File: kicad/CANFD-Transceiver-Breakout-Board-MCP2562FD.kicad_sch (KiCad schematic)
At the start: 15 parts, among them IC1 MCP2562FD-E_SN, K1 HEADER_MALE_6X1, K2 HEADER_MALE_6X1, K3 TERMINAL_KF235-5.0-2P, U3 ATA6561-GAQW-N

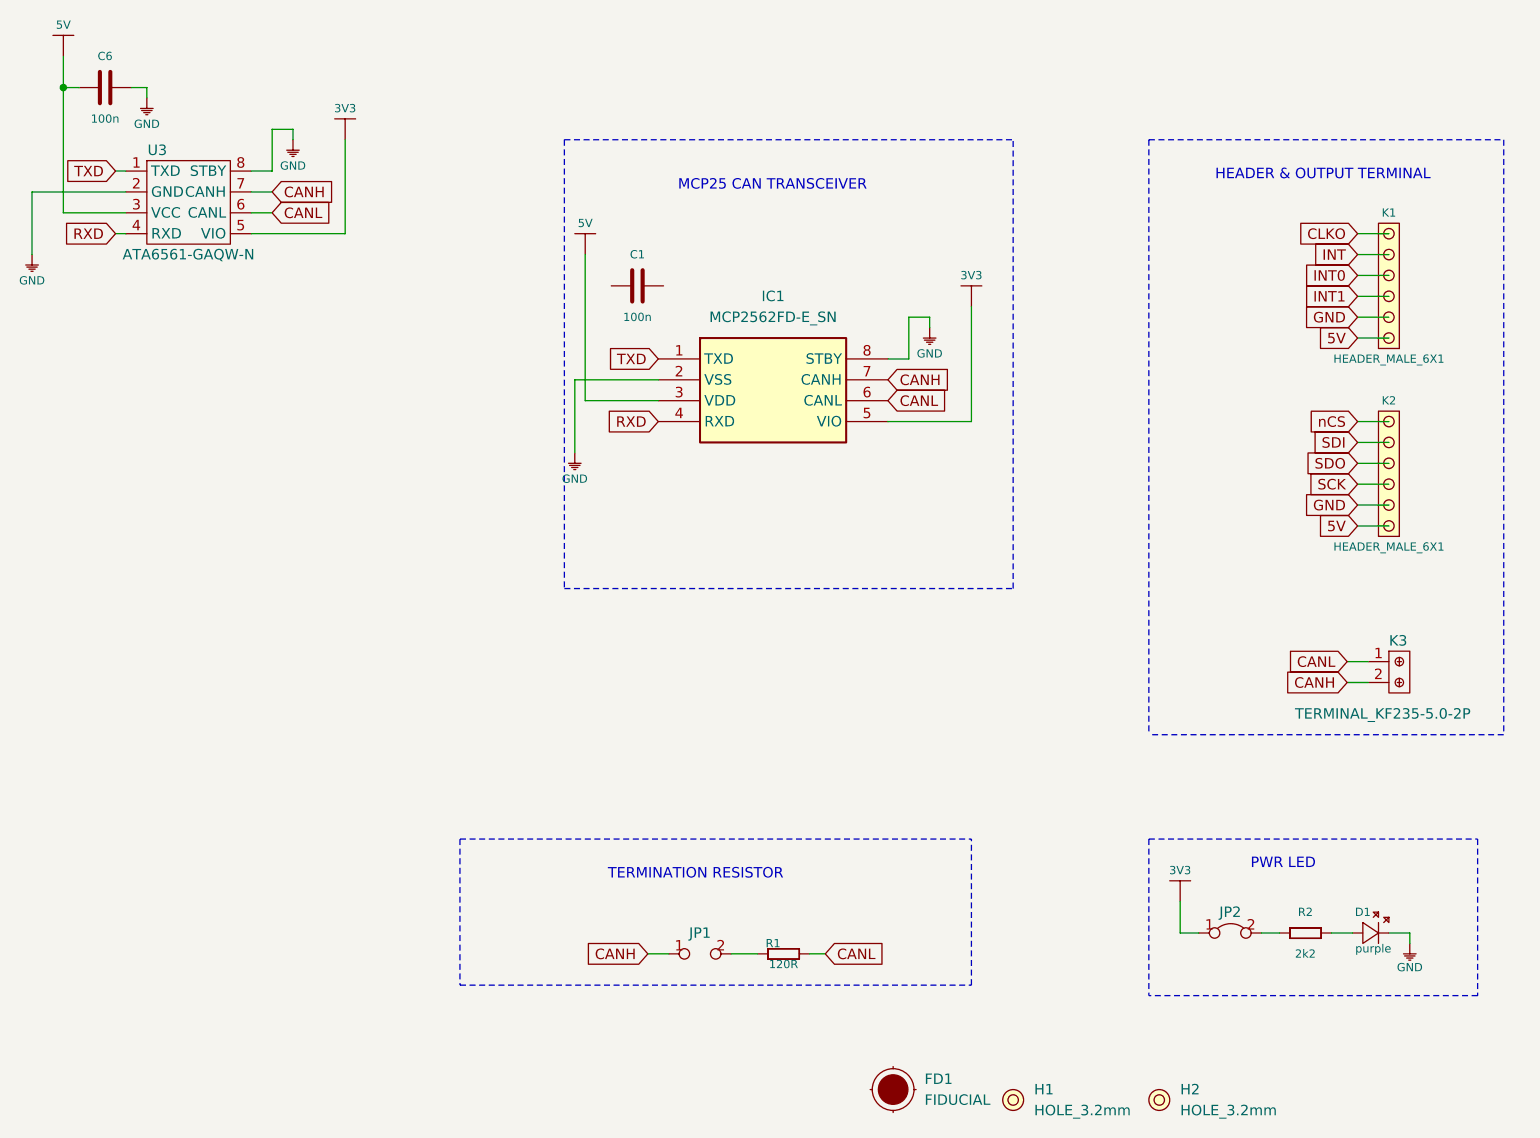
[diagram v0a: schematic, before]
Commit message: editing schematic
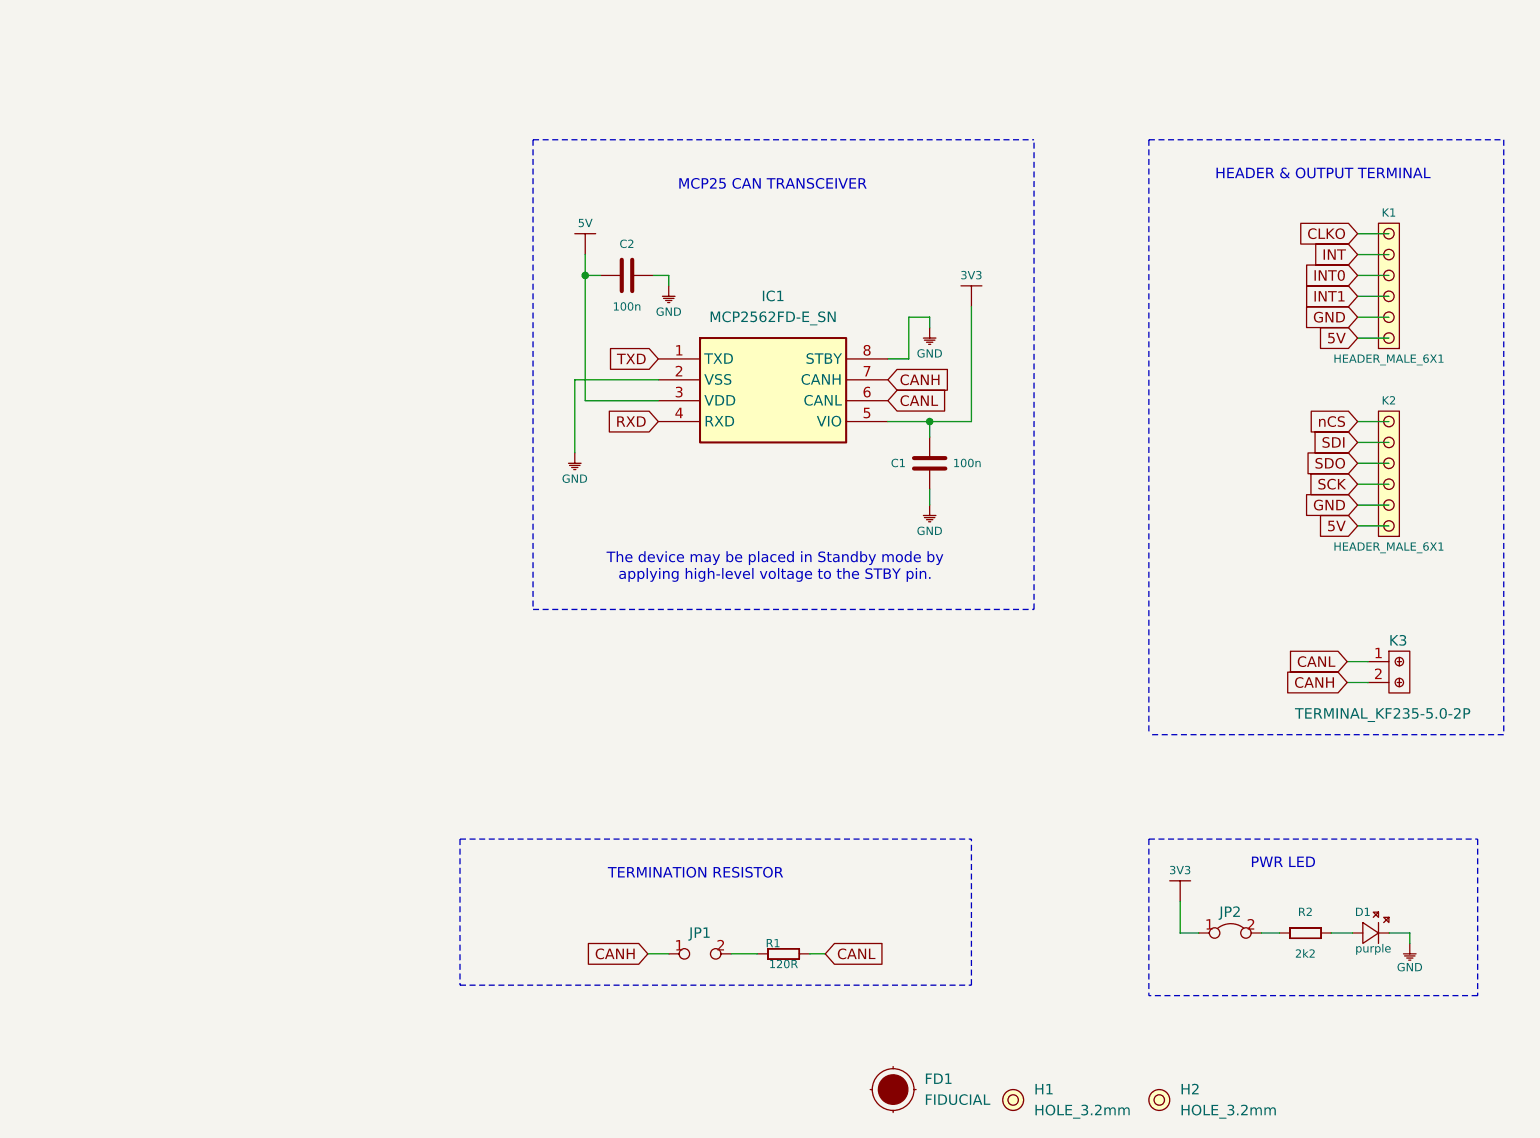
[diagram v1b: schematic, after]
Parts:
- removed C6: 100n, e-radionica.com footprinti:0603C, symbol e-radionica.com schematics:0603C
- removed U3: ATA6561-GAQW-N, e-radionica.com footprinti:SOIC−8, symbol e-radionica.com schematics:ATA6561-GAQW-N
- added C2: 100n, e-radionica.com footprinti:0603C, symbol e-radionica.com schematics:0603C
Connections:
- net 3V3: now also C1.2
- net 5V: now also C2.1
- net GND: now also C1.1, C2.2
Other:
- note added: "The device may be placed in Standby mode by applying high-level voltage to the STBY pin."
